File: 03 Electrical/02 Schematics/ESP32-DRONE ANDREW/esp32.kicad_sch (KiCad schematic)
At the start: 1 part, among them U1 ESP32-C3

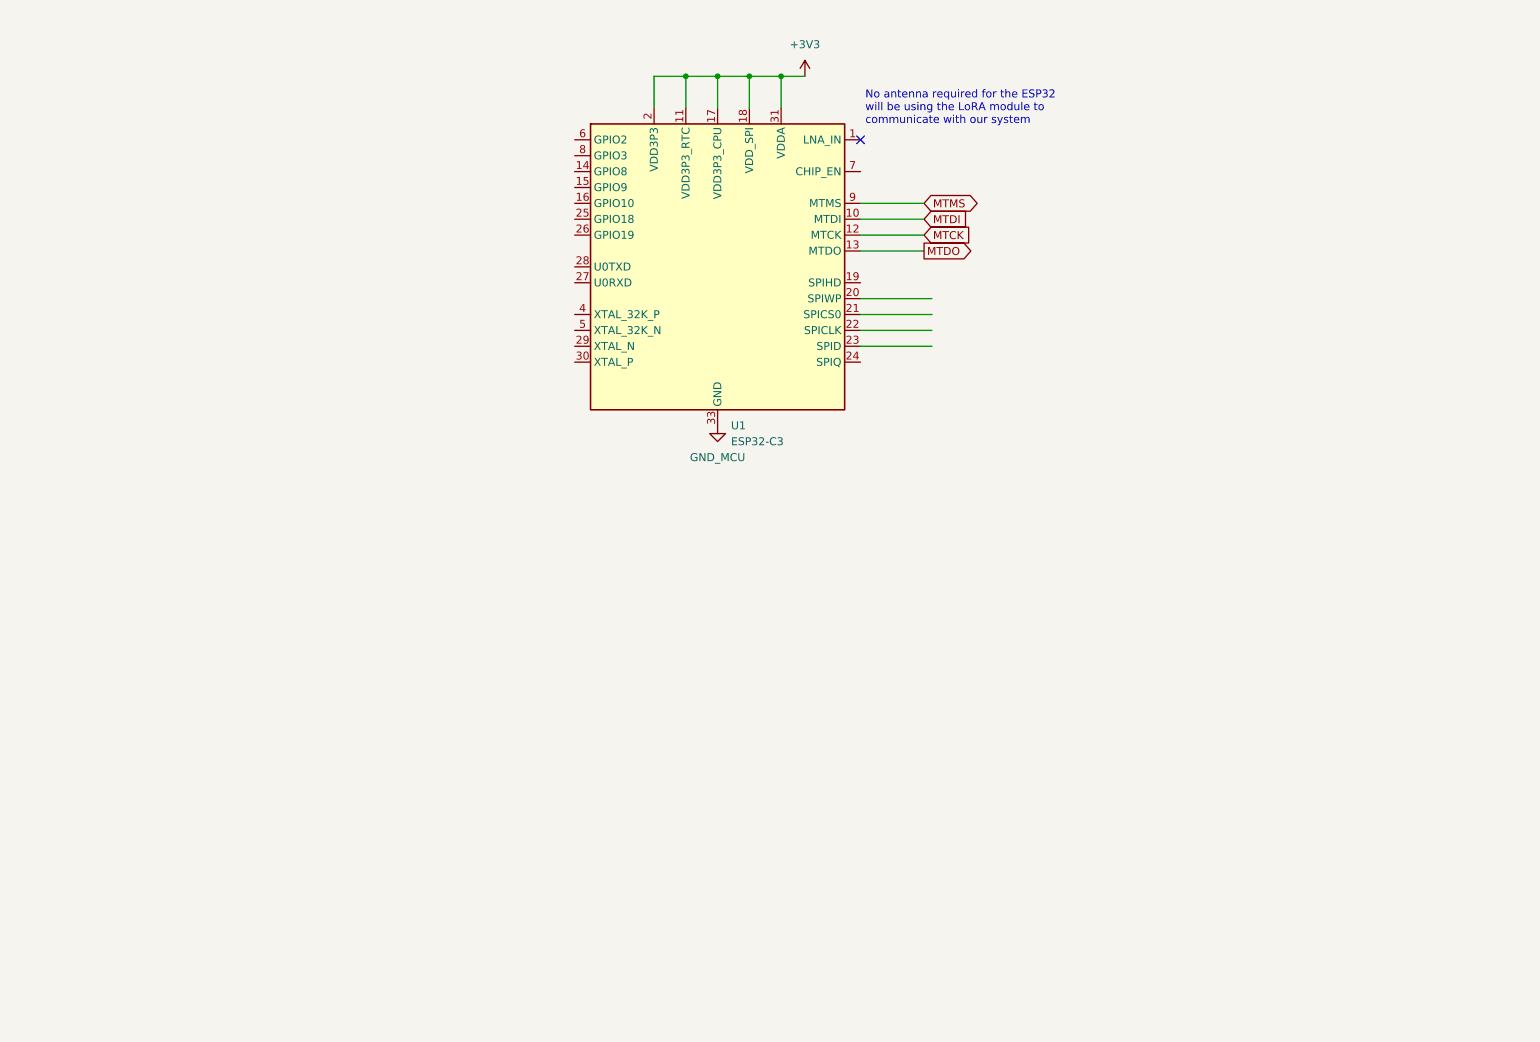
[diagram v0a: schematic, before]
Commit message: finished power managemnt
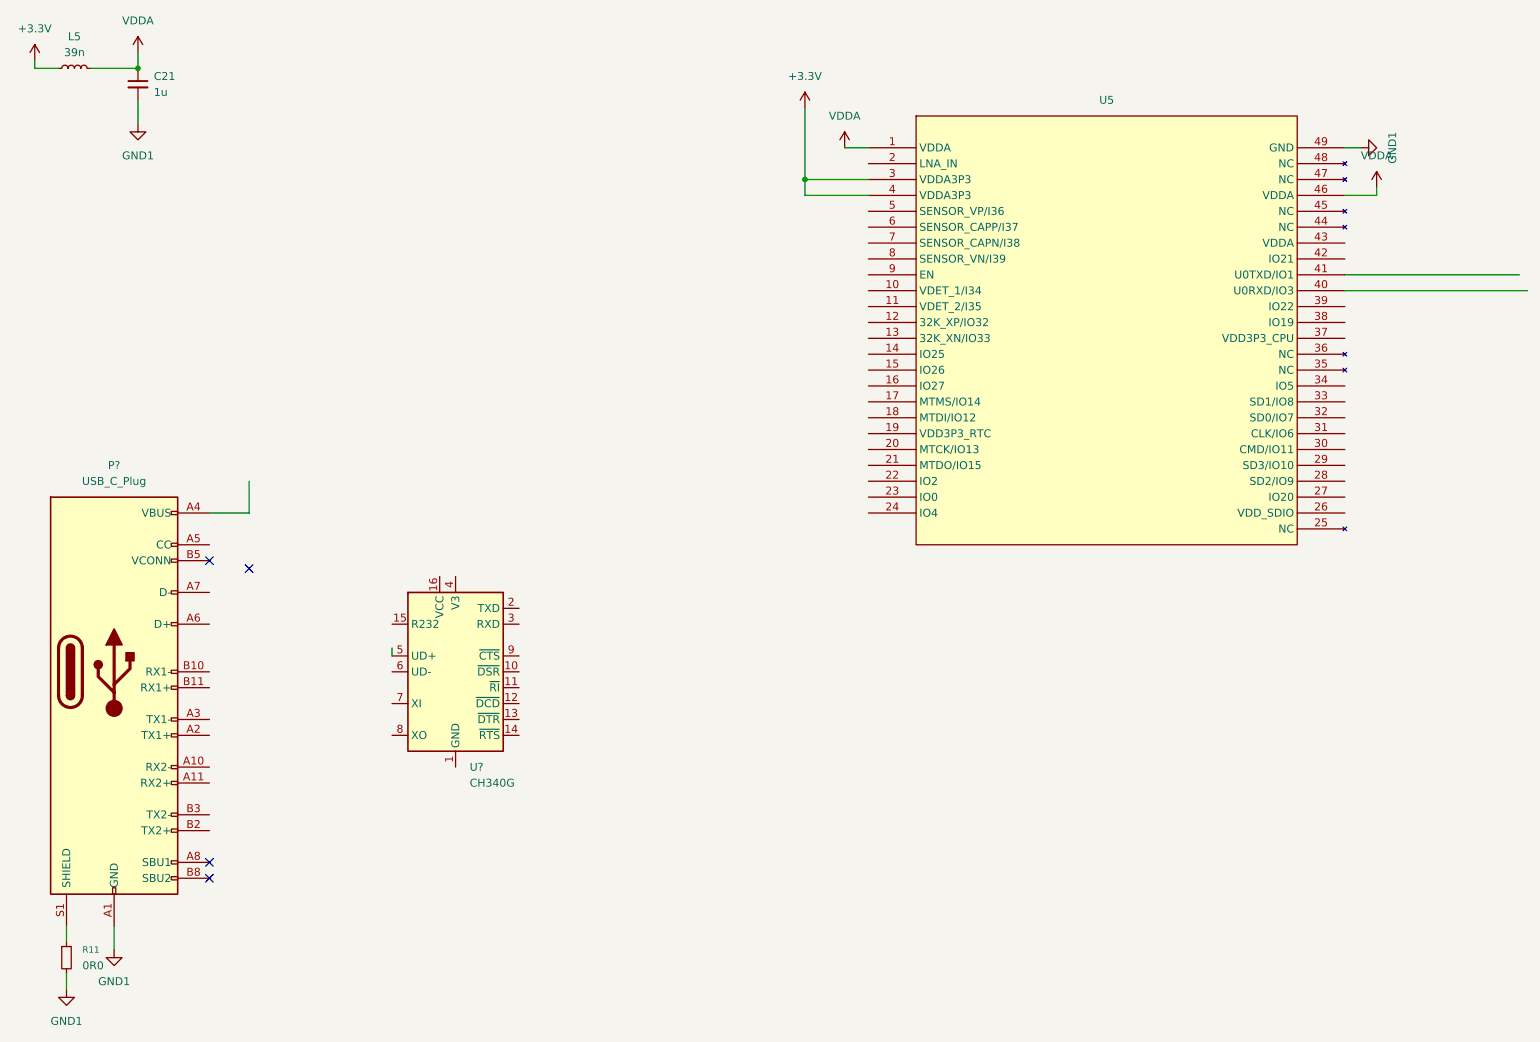
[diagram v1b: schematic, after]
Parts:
- removed U1: ESP32-C3, Package_DFN_QFN:QFN-32-1EP_5x5mm_P0.5mm_EP3.7x3.7mm, symbol MCU_Espressif:ESP32-C3
- added C21: 1u, symbol Device:C_Small
- added L5: 39n, symbol Device:L_Small
- added P?: USB_C_Plug, symbol Connector:USB_C_Plug
- added R11: 0R0, symbol Device:R_Small
- added U5: ~, symbol Library 1:ESP32-PICO-V3
- added U?: CH340G, Package_SO:SOIC-16_3.9x9.9mm_P1.27mm, symbol Interface_USB:CH340G
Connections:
- new net: P?.A4 (VBUS), P?.A9 (VBUS), P?.B4 (VBUS), P?.B9 (VBUS)
- new net: P?.S1 (SHIELD), R11.1
- new net +3.3V: L5.1, U5.3 (VDDA3P3), U5.4 (VDDA3P3)
- new net GND1: C21.2, P?.A1 (GND), P?.A12 (GND), P?.B1 (GND), P?.B12 (GND), R11.2, U5.49 (GND)
- new net VDDA: C21.1, L5.2, U5.1 (VDDA), U5.46 (VDDA)
- no-connect marks 1 -> 4
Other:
- note removed: "No antenna required for the ESP32 will be using the LoRA module to communicate with our system"
